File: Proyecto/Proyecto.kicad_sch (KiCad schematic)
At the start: 19 parts

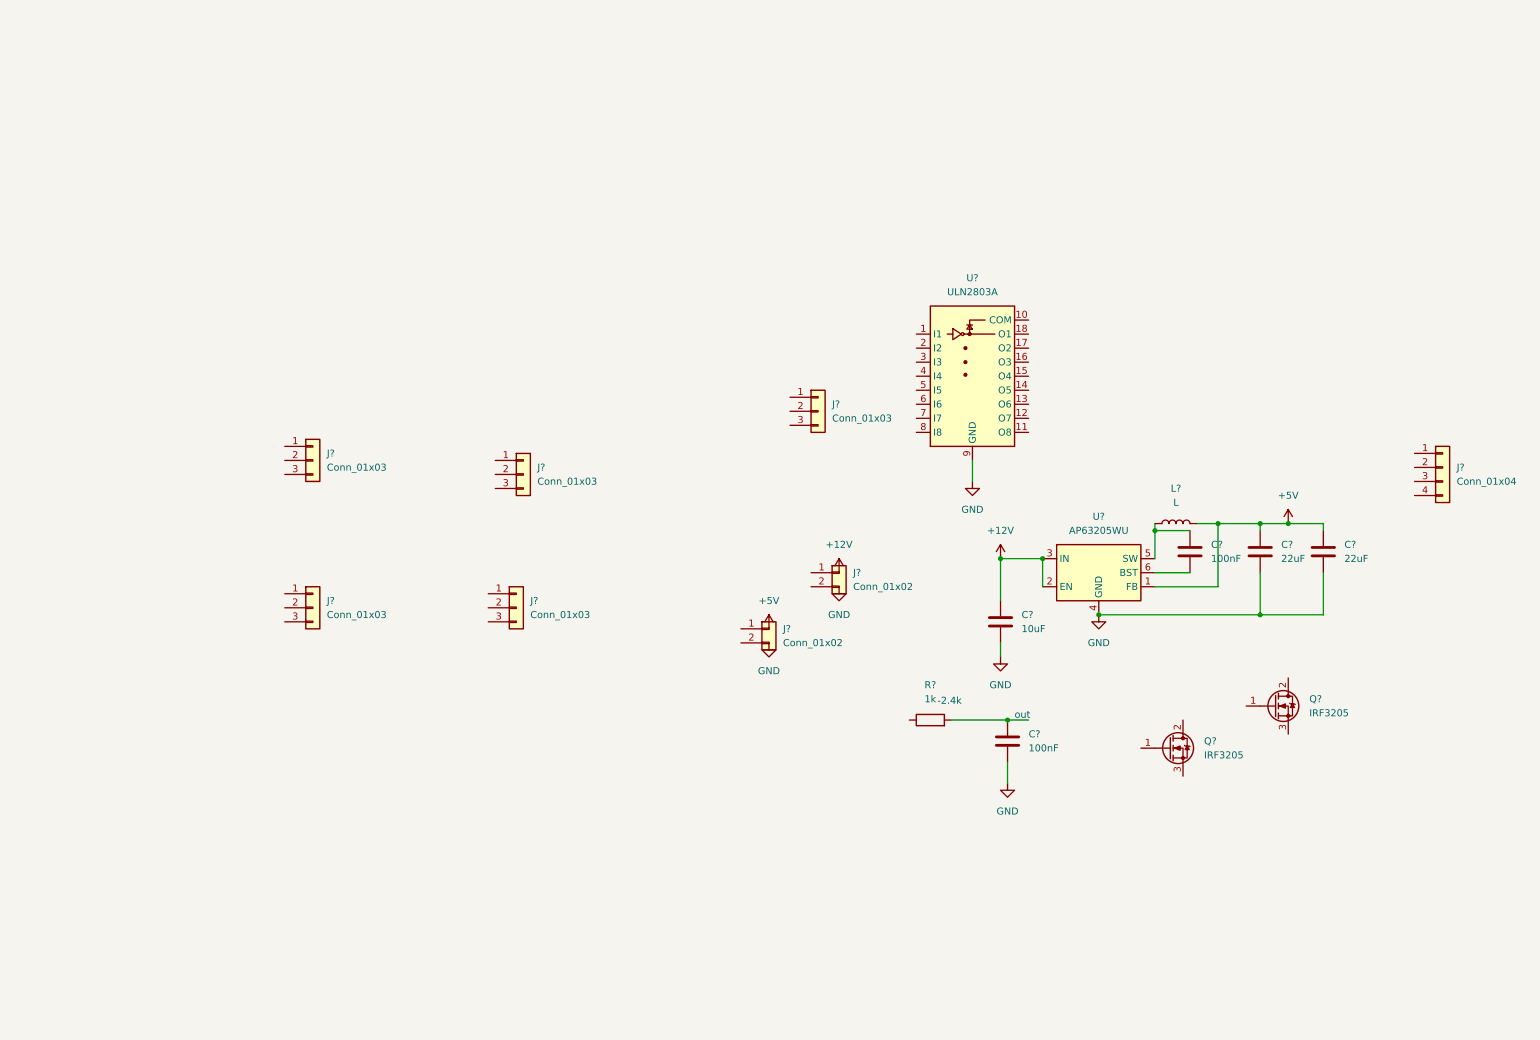
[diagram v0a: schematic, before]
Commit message: 30-6-2022
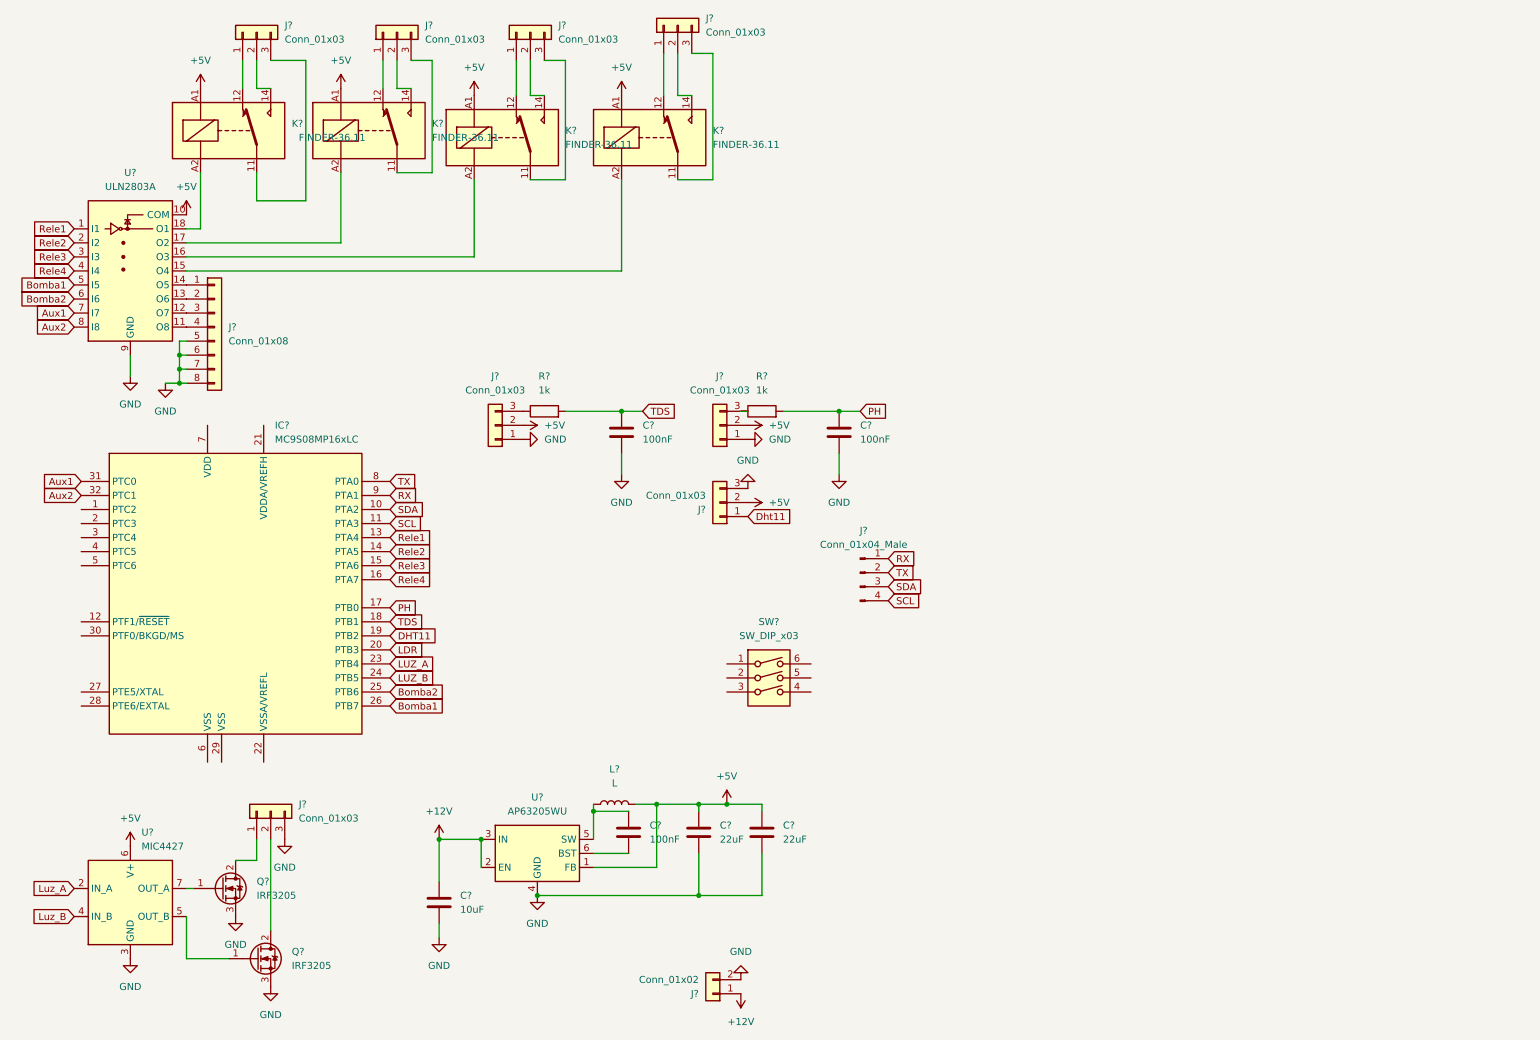
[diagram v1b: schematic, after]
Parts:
- removed J? (x2): Conn_01x03, symbol Connector_Generic:Conn_01x03
- removed J?: Conn_01x04, symbol Connector_Generic:Conn_01x04
- removed J?: Conn_01x02, symbol Connector_Generic:Conn_01x02
- added C?: 100nF, symbol Device:C
- added IC?: MC9S08MP16xLC, Package_QFP:LQFP-32_7x7mm_P0.8mm, symbol MCU_NXP_S08:MC9S08MP16xLC
- added J?: Conn_01x04_Male, symbol Connector:Conn_01x04_Male
- added J? (x5): Conn_01x03, symbol Connector_Generic:Conn_01x03
- added J?: Conn_01x08, symbol Connector_Generic:Conn_01x08
- added K? (x4): FINDER-36.11, Relay_THT:Relay_SPDT_Finder_36.11, symbol Relay:FINDER-36.11
- added R?: 1k, symbol Device:R
- added SW?: SW_DIP_x03, symbol Switch:SW_DIP_x03
- added U?: MIC4427, symbol Driver_FET:MIC4427
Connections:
- net +12V: now also J?.1 (Pin_1)
- net +5V: now also J?.2 (Pin_2), J?.2 (Pin_2), J?.2 (Pin_2), U?.10 (COM), K?.A1, K?.A1, K?.A1, K?.A1, U?.6 (V+)
- net GND: now also J?.1 (Pin_1), J?.1 (Pin_1), J?.2 (Pin_2), J?.3 (Pin_3), Q?.3 (S), Q?.3 (S), C?.2, J?.3 (Pin_3), J?.5 (Pin_5), J?.6 (Pin_6), J?.7 (Pin_7), J?.8 (Pin_8), U?.3 (GND)
- net Rele1: now reaches U?.1 (I1)
- net Rele1: now also IC?.13 (PTA4)
- net at U?.11 (O8): now also J?.4 (Pin_4)
- net at U?.12 (O7): now also J?.3 (Pin_3)
- net at U?.13 (O6): now also J?.2 (Pin_2)
- net at U?.14 (O5): now also J?.1 (Pin_1)
- net at U?.15 (O4): now also K?.A2
- net at U?.16 (O3): now also K?.A2
- net at U?.17 (O2): now also K?.A2
- net at U?.18 (O1): now also K?.A2
- net Rele2: now reaches U?.2 (I2)
- net Rele2: now also IC?.14 (PTA5)
- net Rele3: now reaches U?.3 (I3)
- net Rele3: now also IC?.15 (PTA6)
- net Rele4: now reaches U?.4 (I4)
- net Rele4: now also IC?.16 (PTA7)
- net Bomba1: now reaches U?.5 (I5)
- net Bomba1: now also IC?.26 (PTB7)
- net Bomba2: now reaches U?.6 (I6)
- net Bomba2: now also IC?.25 (PTB6)
- net Aux1: now reaches U?.7 (I7)
- net Aux1: now also IC?.31 (PTC0)
- net Aux2: now reaches U?.8 (I8)
- net Aux2: now also IC?.32 (PTC1)
- net at Q?.1 (G): now also U?.7 (OUT_A)
- net at Q?.2 (D): now also J?.1 (Pin_1)
- net at J?.3 (Pin_3): now also R?.1 (x2)
- net Dht11: now reaches J?.1 (Pin_1)
- net TDS: now reaches C?.1, R?.2
- net TDS: now also IC?.18 (PTB1)
- net at Q?.1 (G): now also U?.5 (OUT_B)
- net at Q?.2 (D): now also J?.2 (Pin_2)
- new net: J?.1 (Pin_1), K?.12 (x4)
- new net: J?.2 (Pin_2), K?.14 (x4)
- new net: J?.3 (Pin_3), K?.11 (x4)
- new net DHT11: IC?.19 (PTB2)
- new net LDR: IC?.20 (PTB3)
- new net LUZ_A: IC?.23 (PTB4)
- new net LUZ_B: IC?.24 (PTB5)
- new net Luz_A: U?.2 (IN_A)
- new net Luz_B: U?.4 (IN_B)
- new net PH: C?.1, IC?.17 (PTB0), R?.2
- new net RX: IC?.9 (PTA1), J?.1 (Pin_1)
- new net SCL: IC?.11 (PTA3), J?.4 (Pin_4)
- new net SDA: IC?.10 (PTA2), J?.3 (Pin_3)
- new net TX: IC?.8 (PTA0), J?.2 (Pin_2)
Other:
- note removed: "-2.4k"
- note removed: "out"
- moved on the sheet: C?, J?, L?, Q?, R?, U?
